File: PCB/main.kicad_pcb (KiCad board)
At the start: 2 copper layers, 76.5 x 37.5 mm, 16 parts, among them J1 USB_C_Receptacle, J2 RJ45, J3 USB_C_Receptacle, J4 USB_C_Receptacle, M1 Fan_PC_Chassis, M2 Fan_PC_Chassis, M3 Fan_PC_Chassis, M4 Fan_PC_Chassis, SW1 SW_DPDT_x2, U2 LAN9512i

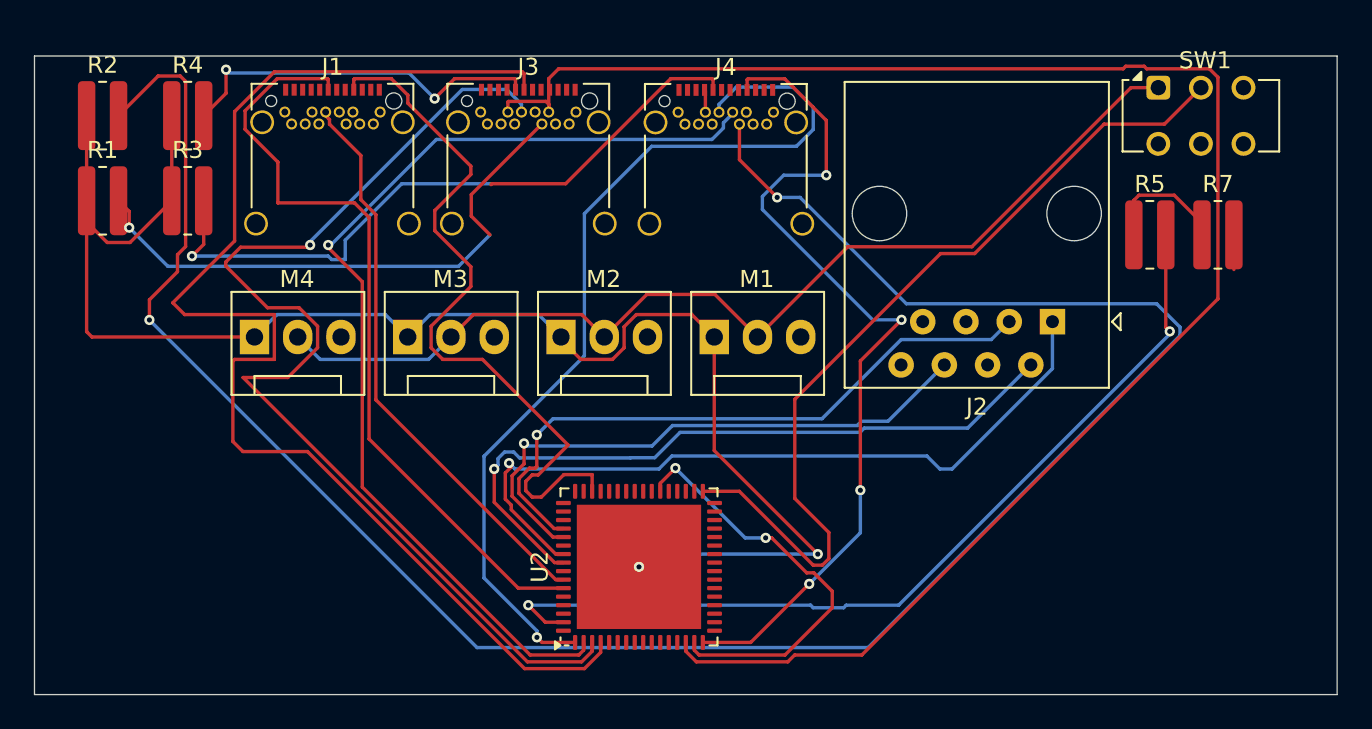
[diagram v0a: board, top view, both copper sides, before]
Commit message: fixing PCB
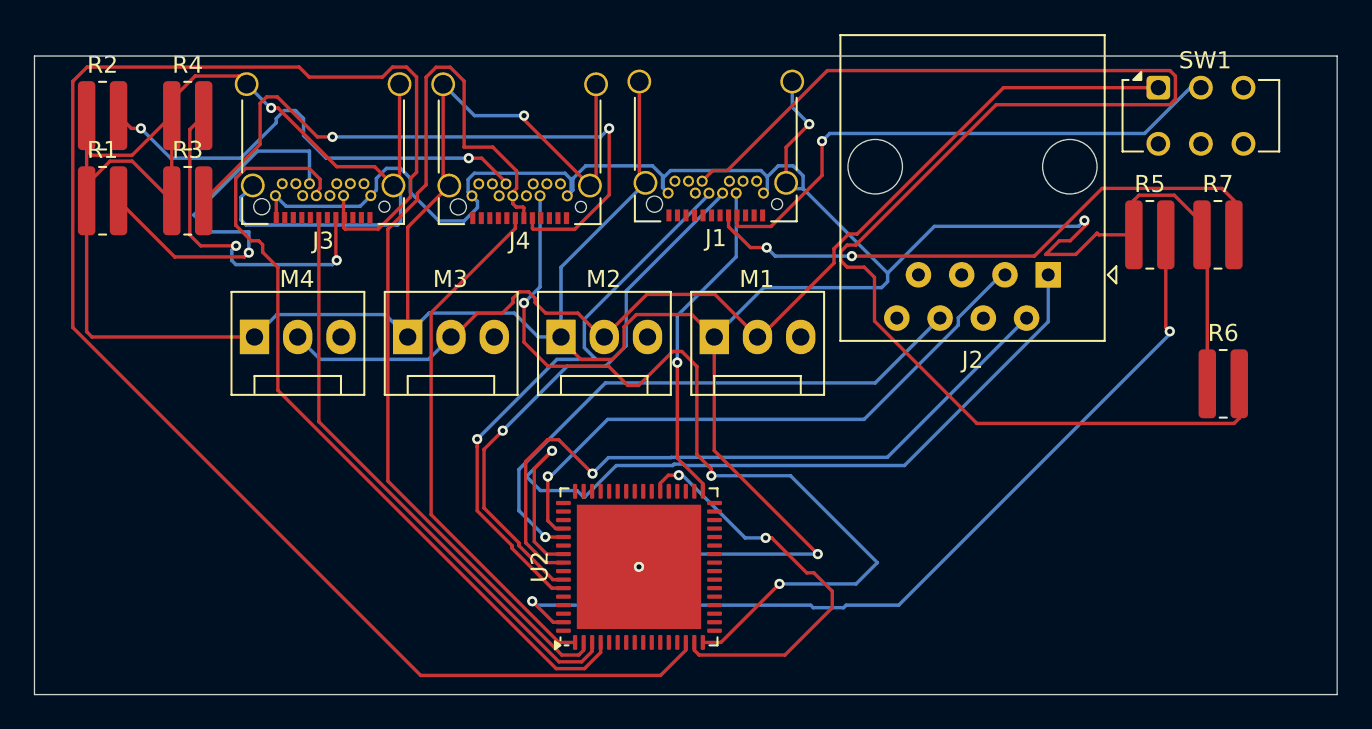
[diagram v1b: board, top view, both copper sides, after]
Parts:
- added R6: R, Resistor_SMD:R_0815_2038Metric, F.Cu at (177.8, 71.8)
- moved J1 22.7 mm to (148.0, 56.8), turned to 180 degrees
- moved J4 12.4 mm to (136.5, 57.0), turned to 180 degrees
- moved J3 12.3 mm to (125.0, 57.0), turned to 180 degrees
- moved J2 2.76 mm to (167.5, 65.3)
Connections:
- J1 pad A5: unconnected-(J1-CC1-PadA5) -> Net-(J1-CC1)
- J1 pad B5: unconnected-(J1-CC2-PadB5) -> Net-(J1-CC2)
- J1 pad S1: unconnected-(J1-SHIELD-PadS1) -> gnd
- J3 pad S1: unconnected-(J3-SHIELD-PadS1) -> gnd
- J4 pad S1: unconnected-(J4-SHIELD-PadS1) -> gnd
- R7 pad 2: unconnected-(R7-Pad2) -> Net-(J1-CC1)
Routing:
- net gnd: track 101.2 -> 301.4 mm, vias 2 -> 6
- net Net-(J4-CC2): track 128.5 -> 27.5 mm
- net Net-(J1-CC2): track 0.00 -> 86.9 mm
- net VBUSUP: track 94.2 -> 52.0 mm, vias 0 -> 2
- net Net-(J1-CC1): track 0.00 -> 35.0 mm, vias 0 -> 2
- net D-DOWN2: track 64.1 -> 34.6 mm, vias 1 -> 0
- net D+DOWN2: track 75.9 -> 47.0 mm
- net D-DOWN1: track 54.7 -> 31.0 mm, vias 1 -> 0
- net D+UP: track 46.3 -> 33.2 mm, vias 0 -> 1
- net Net-(J3-CC2): track 33.4 -> 24.3 mm
- net D+DOWN1: track 59.9 -> 54.7 mm, vias 1 -> 0
- net Net-(U2B-PRTCTL2): track 99.2 -> 95.1 mm
- net Net-(U2B-TXP): track 45.1 -> 48.2 mm
- net Net-(U2B-RXP): track 38.0 -> 35.7 mm
- net unconnected-(R7-Pad2): track 2.04 -> 0.00 mm
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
